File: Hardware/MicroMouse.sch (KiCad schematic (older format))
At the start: 1 part

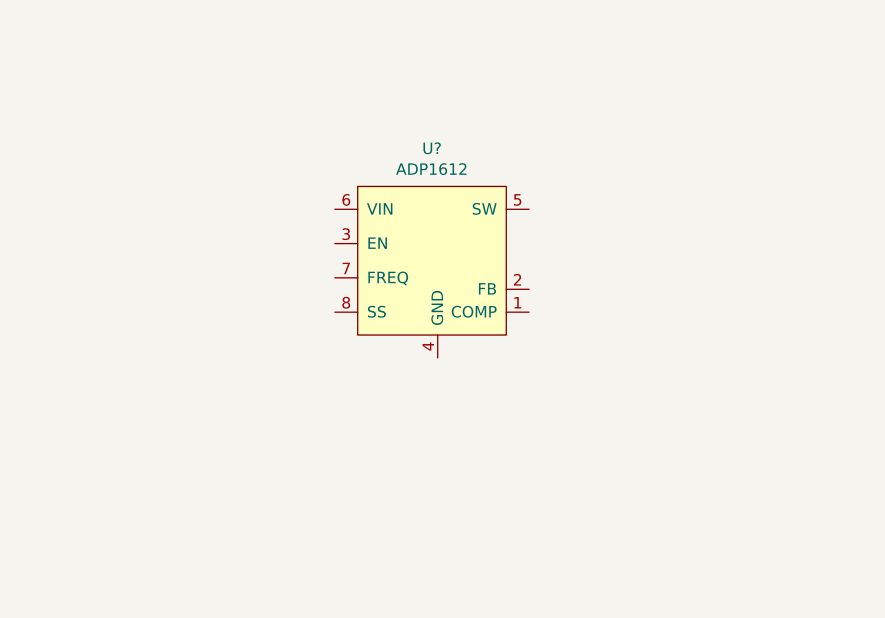
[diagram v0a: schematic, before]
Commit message: Added Power Managemen Dsign
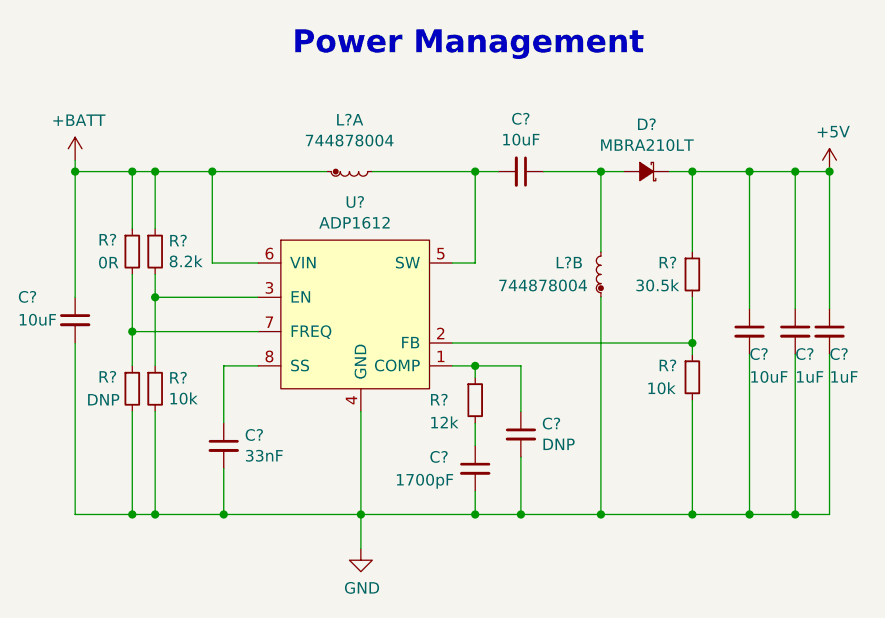
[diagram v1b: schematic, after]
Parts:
- added C? (x3): 10uF, symbol Device:C_Small
- added C?: 1700pF, symbol Device:C_Small
- added C?: DNP, symbol Device:C_Small
- added C? (x2): 1uF, symbol Device:C_Small
- added C?: 33nF, symbol Device:C_Small
- added D?: MBRA210LT, symbol Device:D_Schottky_Small_ALT
- added L? (x2): 744878004, symbol Mice_Sym:744878004
- added R?: 8.2k, symbol Device:R_Small
- added R?: 0R, symbol Device:R_Small
- added R? (x2): 10k, symbol Device:R_Small
- added R?: DNP, symbol Device:R_Small
- added R?: 12k, symbol Device:R_Small
- added R?: 30.5k, symbol Device:R_Small
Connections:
- net at U?.1 (COMP): now also C?.1, R?.1
- net at U?.2 (FB): now also R?.1, R?.2
- net at U?.3 (EN): now also R?.1, R?.2
- net GND: now reaches U?.4 (GND)
- net GND: now also C?.2, C?.2, C?.2, C?.2, C?.2, C?.2, C?.2, L?.4, R?.2, R?.2, R?.2
- net at U?.5 (SW): now also C?.2, L?.2
- net +BATT: now reaches U?.6 (VIN)
- net +BATT: now also C?.1, L?.1, R?.1, R?.1
- net at U?.7 (FREQ): now also R?.1, R?.2
- net at U?.8 (SS): now also C?.1
- new net: C?.1, D?.2 (A), L?.3
- new net: C?.1, R?.2
- new net +5V: C?.1, C?.1, C?.1, D?.1 (K), R?.1
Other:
- note added: "Power Management"
- moved on the sheet: U?
